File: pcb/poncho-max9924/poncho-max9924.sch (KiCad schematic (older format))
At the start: 48 parts, among them J1 Screw_Terminal_01x02, J2 Screw_Terminal_01x02, J3 jumper_4_open, U1 MAX9924, U2 MAX9000

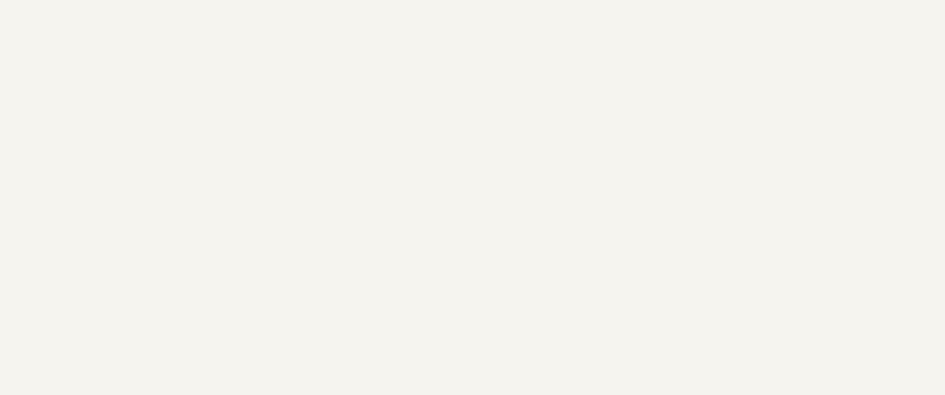
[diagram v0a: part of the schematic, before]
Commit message: primer routeado
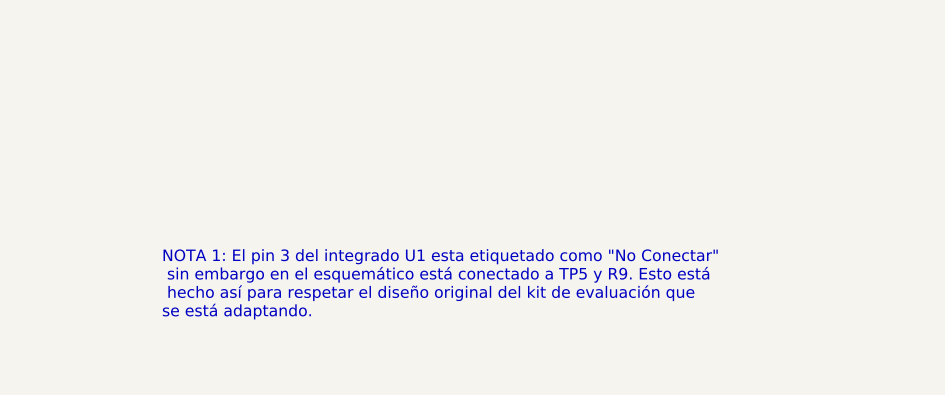
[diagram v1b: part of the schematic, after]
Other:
- note added: "NOTA 1: El pin 3 del integrado U1 esta etiquetado como "No Conectar"\n sin embargo en el esquemático está conectado a TP5 y R9. Esto está\n hecho así para respetar el diseño original del kit de evaluación que \nse está adaptando."
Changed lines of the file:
@@
 	0    1    1    0
 $EndComp
+Text Notes 8400 6500 0    50   ~ 0
+NOTA 1: El pin 3 del integrado U1 esta etiquetado como "No Conectar"\n sin embargo en el esquemático está conectado a TP5 y R9. Esto está\n hecho así para respetar el diseño original del kit de evaluación que \nse está adaptando.
 $EndSCHEMATC
